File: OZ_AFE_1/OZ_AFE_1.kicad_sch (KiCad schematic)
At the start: 57 parts, among them U1 LT6011, U2 TLV2211, U4 LT6011, U5 OGS, U6 MCP9700x-HTT, U7 REF35250QDBVR

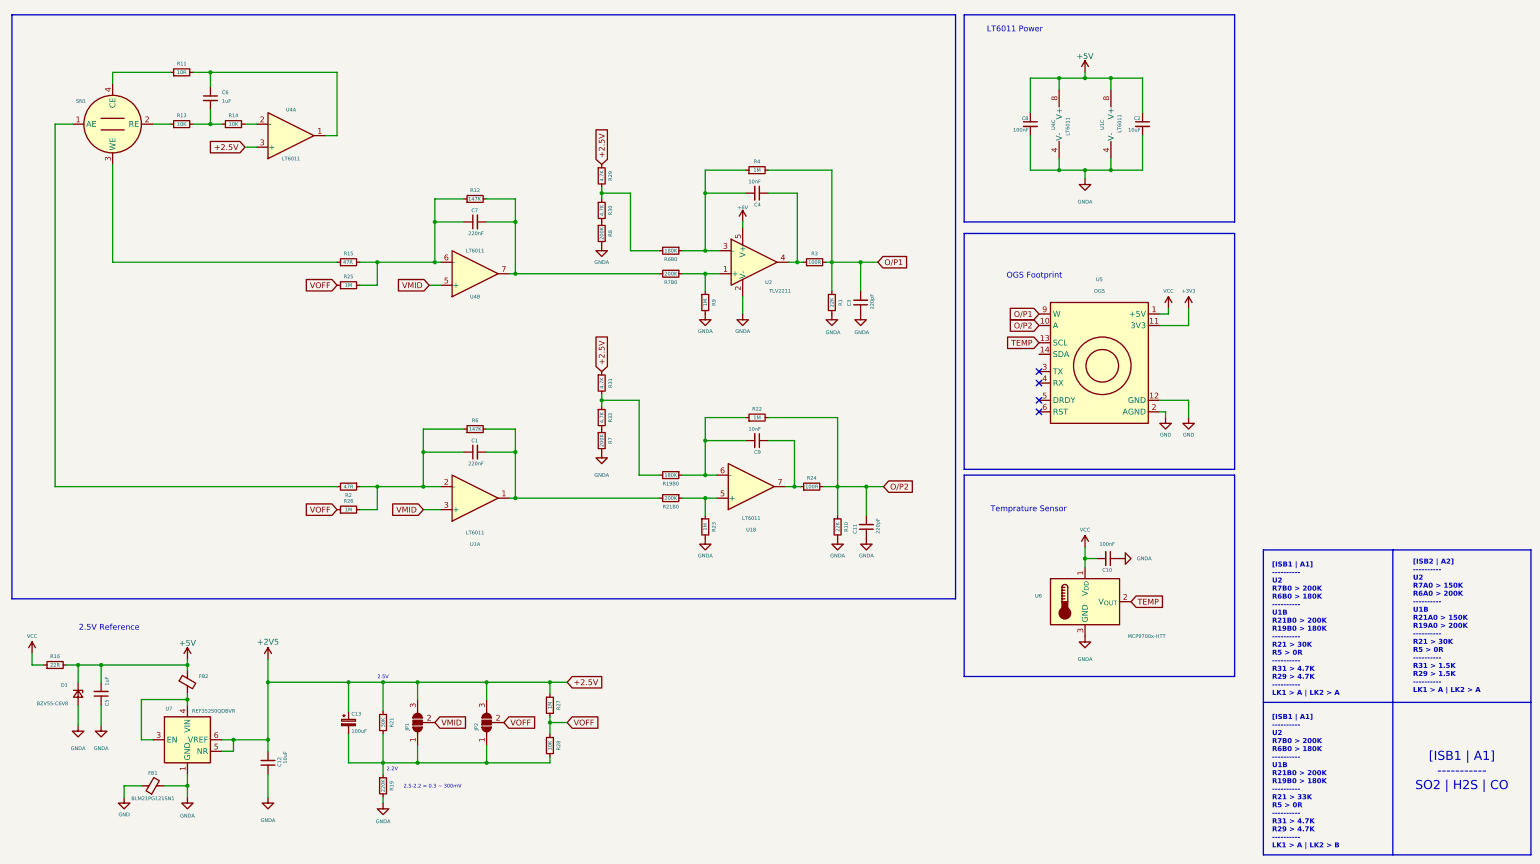
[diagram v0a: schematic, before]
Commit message: sch update
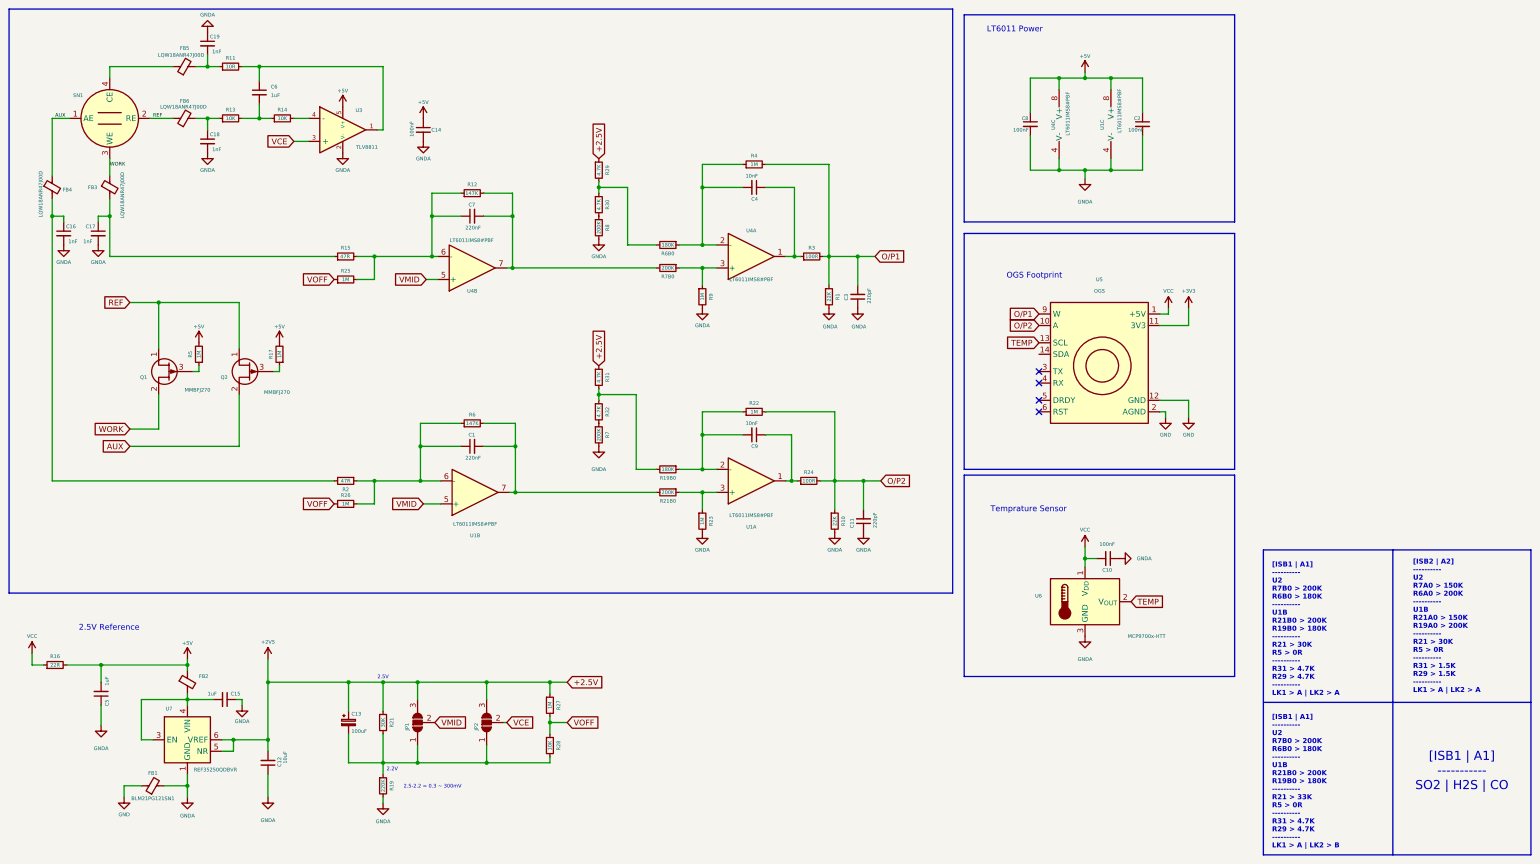
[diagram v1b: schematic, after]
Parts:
- removed D1: BZV55-C6V8, Diode_SMD:D_MiniMELF, symbol Device:D_Zener_Small
- removed U2: TLV2211, Package_TO_SOT_SMD:SOT-23-5, symbol Operational-Amplifiers:TLV2211
- added C14: 100nF, Capacitor_SMD:C_0603_1608Metric, symbol Device:C_Small
- added C15: 1uF, Capacitor_SMD:C_0603_1608Metric, symbol Device:C_Small
- added C16, C17, C18, C19: 1nF, Capacitor_SMD:C_0402_1005Metric, symbol Device:C_Small
- added FB3, FB4, FB5, FB6: LQW18ANR47J00D, Inductor_SMD:L_0603_1608Metric, symbol Device:FerriteBead_Small
- added Q1, Q2: MMBFJ270, Package_TO_SOT_SMD:SOT-23, symbol Device:Q_PJFET_DSG
- added R17, R5: 1M, Resistor_SMD:R_0402_1005Metric, symbol Device:R_Small
- added U3: TLV8811, Package_TO_SOT_SMD:SOT-23-6, symbol TLV8811:TLV8811
- C2: value 10uF -> 100nF
- FB1, FB2: footprint (none) -> Resistor_SMD:R_0805_2012Metric
- JP1, JP2: footprint (none) -> Jumper:SolderJumper-3_P1.3mm_Open_RoundedPad1.0x1.5mm
- R1, R10, R13, R14, R15, R2, R22, R23, R24, R25, R26, R27, R28, R3, R4, R9: footprint Resistor_SMD:R_0603_1608Metric -> Resistor_SMD:R_0402_1005Metric
- U1, U4: value LT6011 -> LT6011IMS8#PBF; footprint Package_SO:SOIC-8_3.9x4.9mm_P1.27mm -> Package_SO:MSOP-8_3x3mm_P0.65mm
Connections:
- net +2V5: no longer U4.3 (+)
- net +5V: now also C14.1, R17.2, R5.2, U3.5 (V+)
- net GNDA: now also C14.2, C15.1, C16.2, C17.2, C18.2, C19.1, U3.2 (V-)
- net VMID: now also U1.5 (+); no longer U1.3 (+)
- net VOFF: no longer JP2.2 (C)
- net at C4.2, R4.1, R6B0.1: now also U4.2 (-)
- net at R21B0.1, R23.1: now also U1.3 (+); no longer U1.5 (+)
- net at C9.2, R19B0.1, R22.1: now also U1.2 (-); no longer U1.6 (-)
- net at C9.1, R24.1: now also U1.1; no longer U1.7
- net at R15.1: now also C17.1, FB3.2; no longer SN1.3 (WE)
- net at C4.1, R3.1: now also U4.1
- net at C1.1, R2.1, R26.2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: now also U1.6 (-); no longer U1.2 (-)
- net at R2.2: now also C16.1, FB4.2; no longer SN1.1 (AE)
- net at FB2.2, U7.3 (EN), U7.4 (VIN): now also C15.2
- net at C1.2, R21B0.2, R6.2: now also U1.7; no longer U1.1
- net at R11.1: now also C19.2, FB5.2; no longer SN1.4 (CE)
- net at C6.1, R11.2: now also U3.1; no longer U4.1
- net at R7B0.1, R9.1: now also U4.3 (+)
- net at R13.1: now also C18.1, FB6.2; no longer SN1.2 (RE)
- net at R14.2: now also U3.4 (-); no longer U4.2 (-)
- new net: Q1.3 (G), R5.1
- new net: FB5.1, SN1.4 (CE)
- new net: Q2.3 (G), R17.1
- new net AUX: FB4.1, Q2.2 (S), SN1.1 (AE)
- new net REF: FB6.1, Q1.1 (D), Q2.1 (D), SN1.2 (RE)
- new net VCE: JP2.2 (C), U3.3 (+)
- new net WORK: FB3.1, Q1.2 (S), SN1.3 (WE)
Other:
- moved on the sheet: C1, C11, C3, C4, C6, C7, C9, R1, R10, R11, R12, R13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
